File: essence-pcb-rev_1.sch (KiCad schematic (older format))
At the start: 133 parts

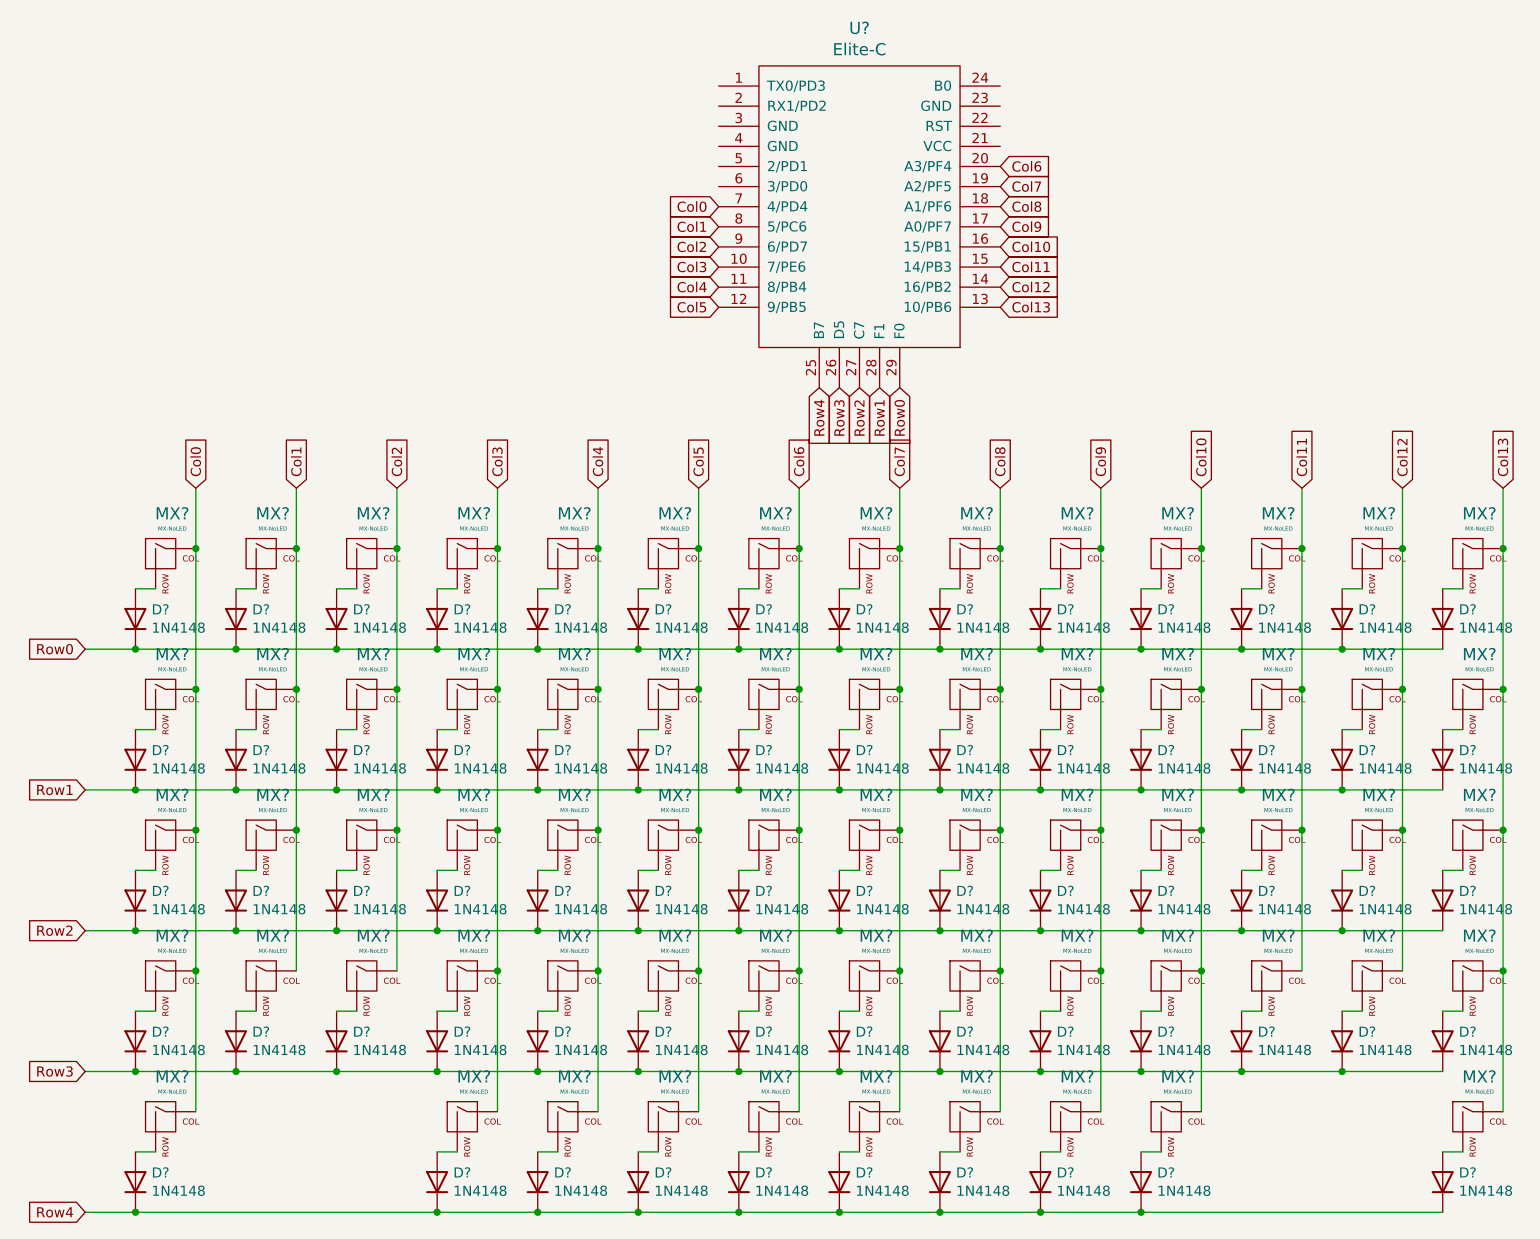
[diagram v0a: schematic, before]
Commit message: Annotations for schematic components
I now need to look for a footprint for the Rotary Encoder, although I think I found it off of the KiCad Subreddit. If you are reading this for some reason, random person, go make a sandwich.
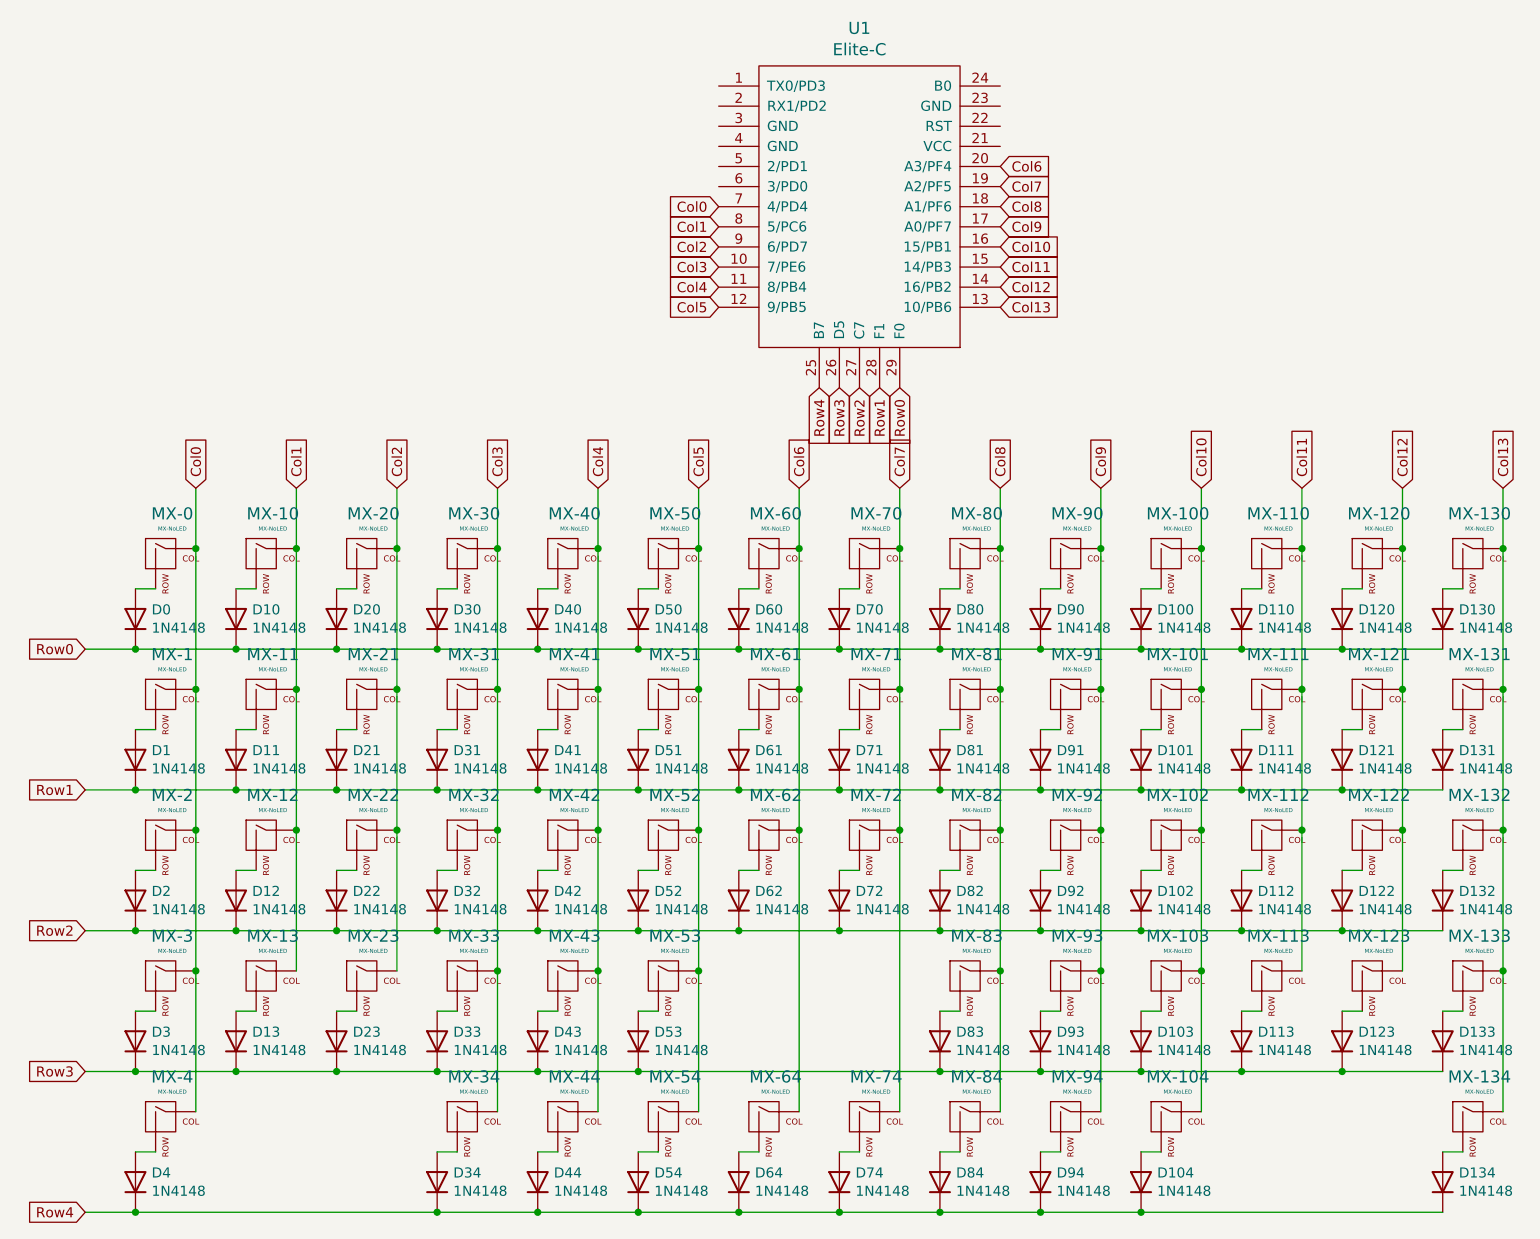
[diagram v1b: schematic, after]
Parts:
- removed D? (x2): 1N4148, Diode_THT:D_DO-35_SOD27_P7.62mm_Horizontal, symbol Diode:1N4148
- removed MX? (x2): MX-NoLED, symbol MX_Alps_Hybrid:MX-NoLED
- gave numbers to parts that had none: 129
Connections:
- net Row3: no longer D64.1 (K), D74.1 (K)
- net Row4: now also D64.1 (K), D74.1 (K)
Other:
- moved on the sheet: D64, D74, MX-64, MX-74
